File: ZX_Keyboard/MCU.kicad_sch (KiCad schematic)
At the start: 19 parts, among them J1 DBG_UART, J2 DEBUG, SW1 RESET, U1 STM32F105R8Tx, Y1 8MHz

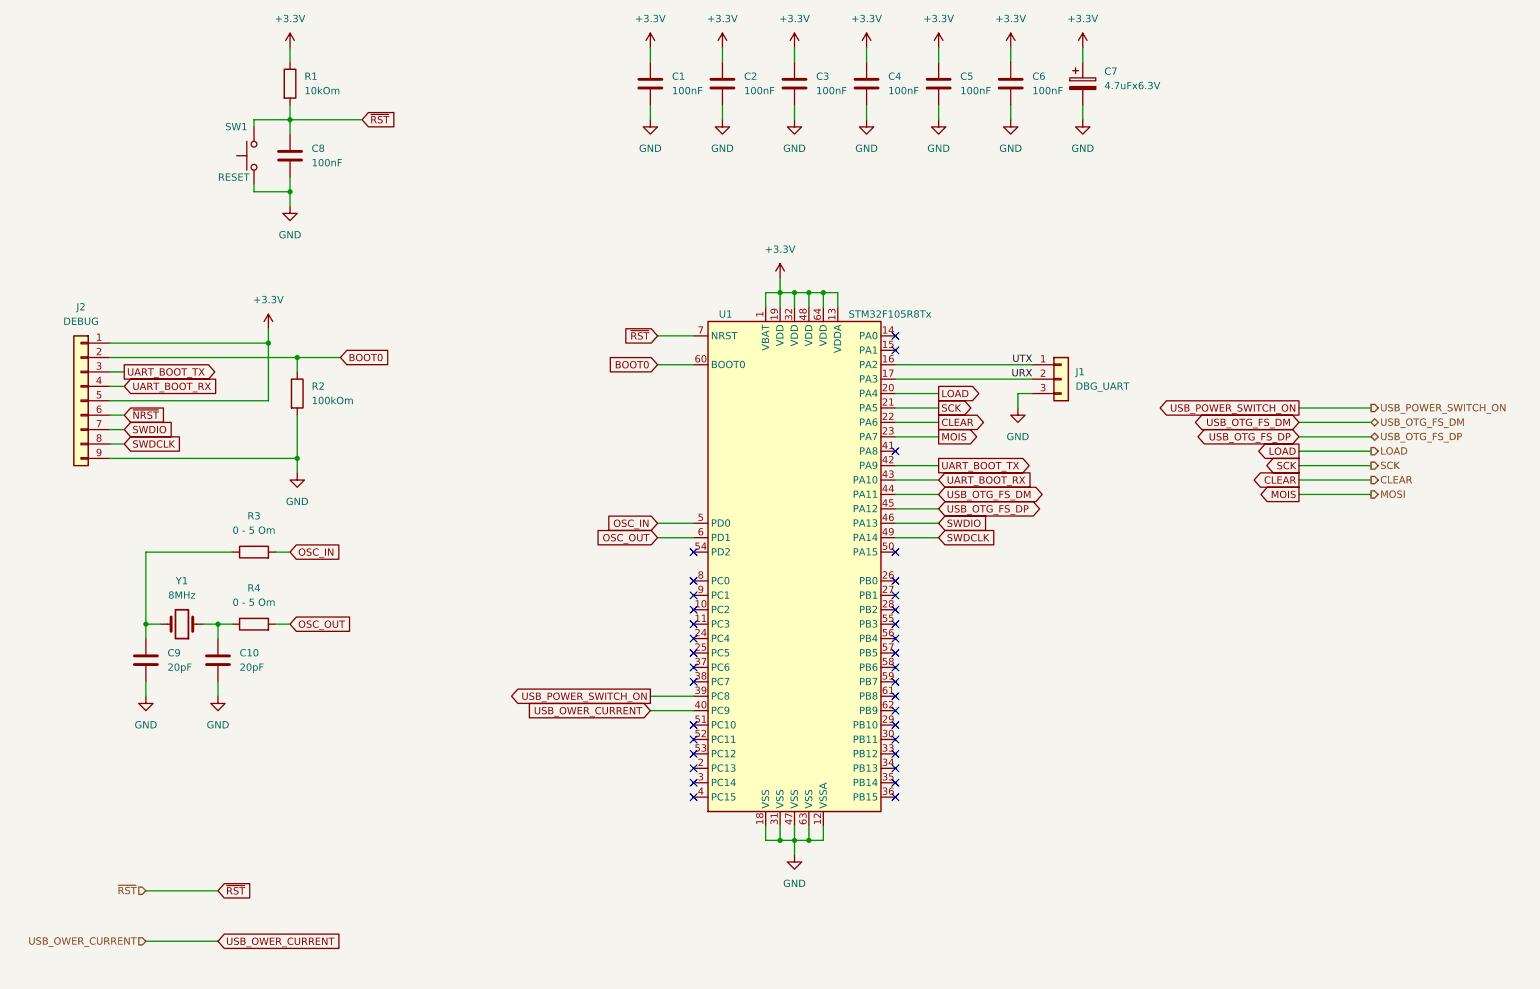
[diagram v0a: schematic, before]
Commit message: update and fix schematic
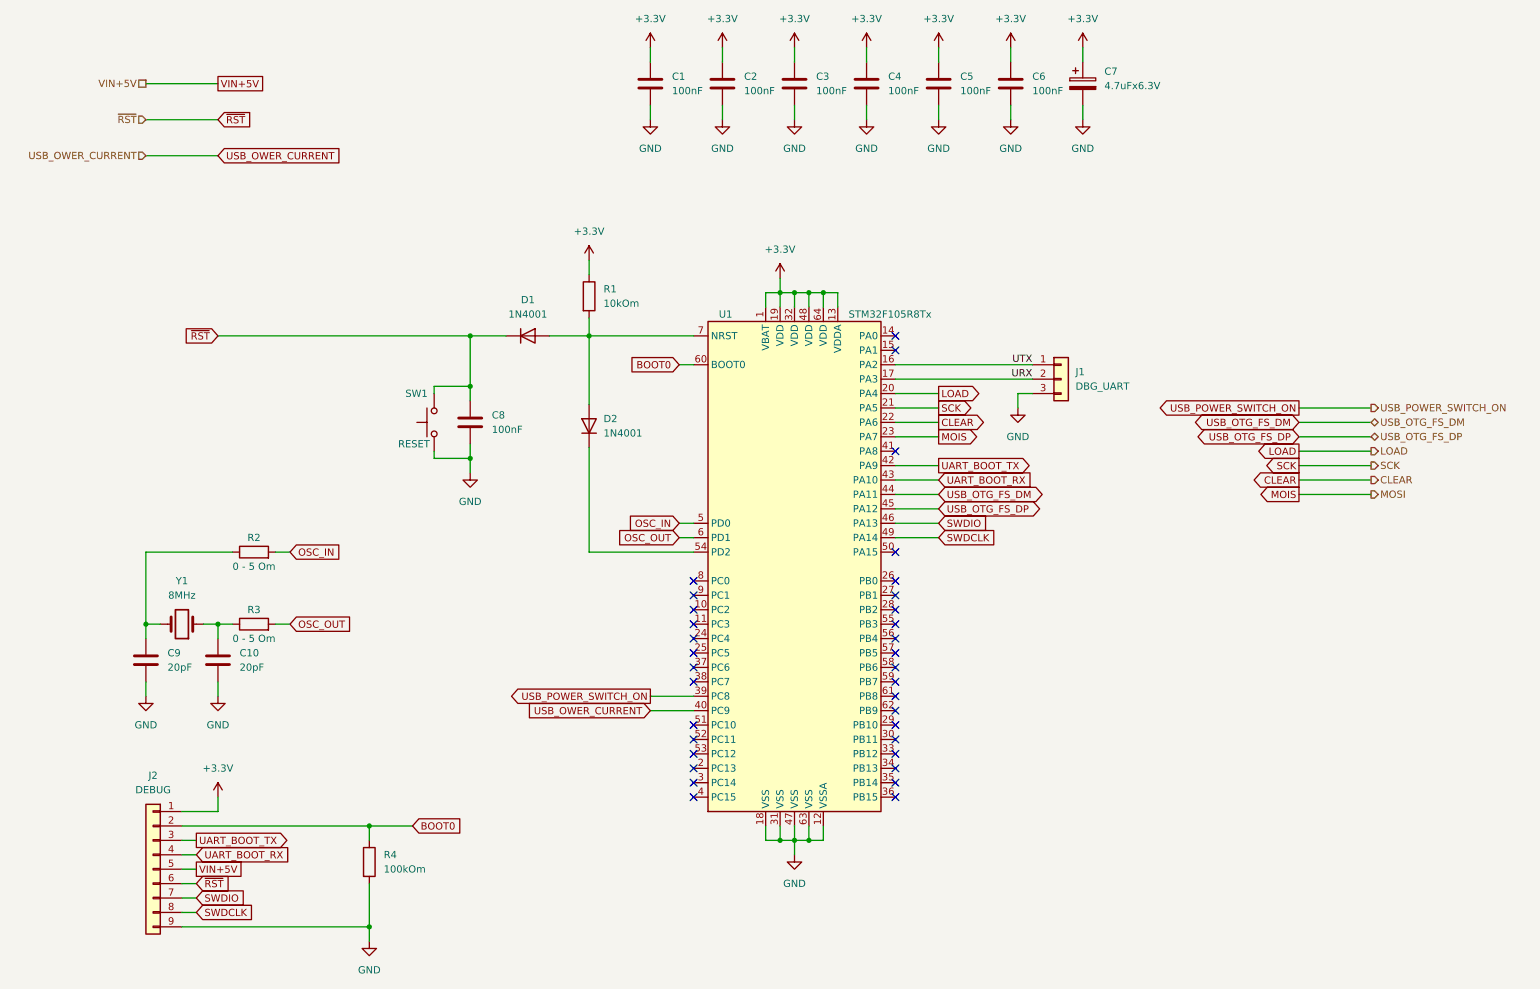
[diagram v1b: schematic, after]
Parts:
- added D1, D2: 1N4001, symbol Device:D
- renumbered R3 to R2, R4 to R3, R2 to R4
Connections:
- net ~{NRST} is gone; now on net ~{RST}: J2.6 (Pin_6)
- net +3.3V: no longer J2.5 (Pin_5)
- net ~{RST}: now also D1.1 (K); no longer R1.2, U1.7 (NRST)
- net at U1.54 (PD2): now also D2.1 (K)
- new net: D1.2 (A), D2.2 (A), R1.2, U1.7 (NRST)
- new net VIN+5V: J2.5 (Pin_5)
- no-connect marks 35 -> 34
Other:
- moved on the sheet: C8, J2, R1, R4, SW1
